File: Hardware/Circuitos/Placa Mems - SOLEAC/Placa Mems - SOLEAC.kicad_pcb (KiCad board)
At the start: 2 copper layers, 50 x 40 mm, 7 parts, among them J2 Conn_01x04, J6 Conn_01x02, Y1 MA40S4R

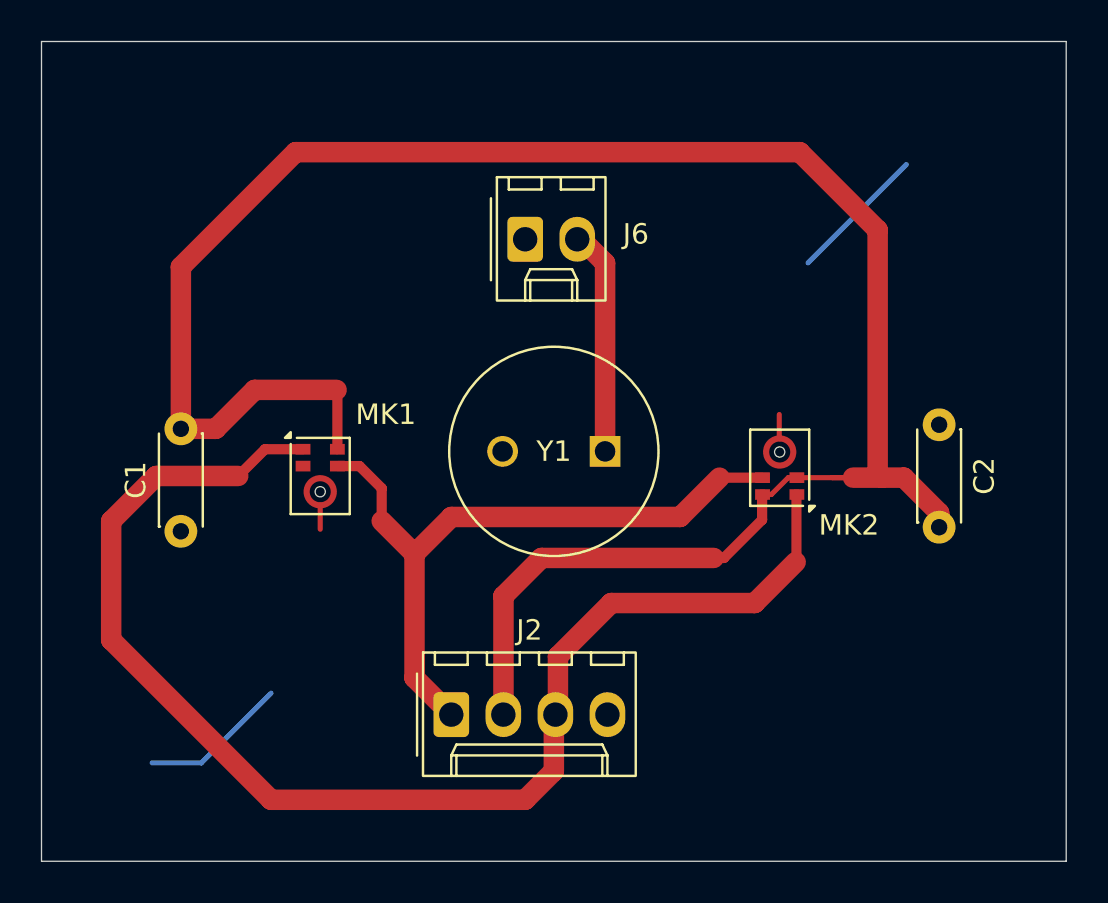
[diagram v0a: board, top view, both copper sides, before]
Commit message: Placa Mems - Zona de tierra
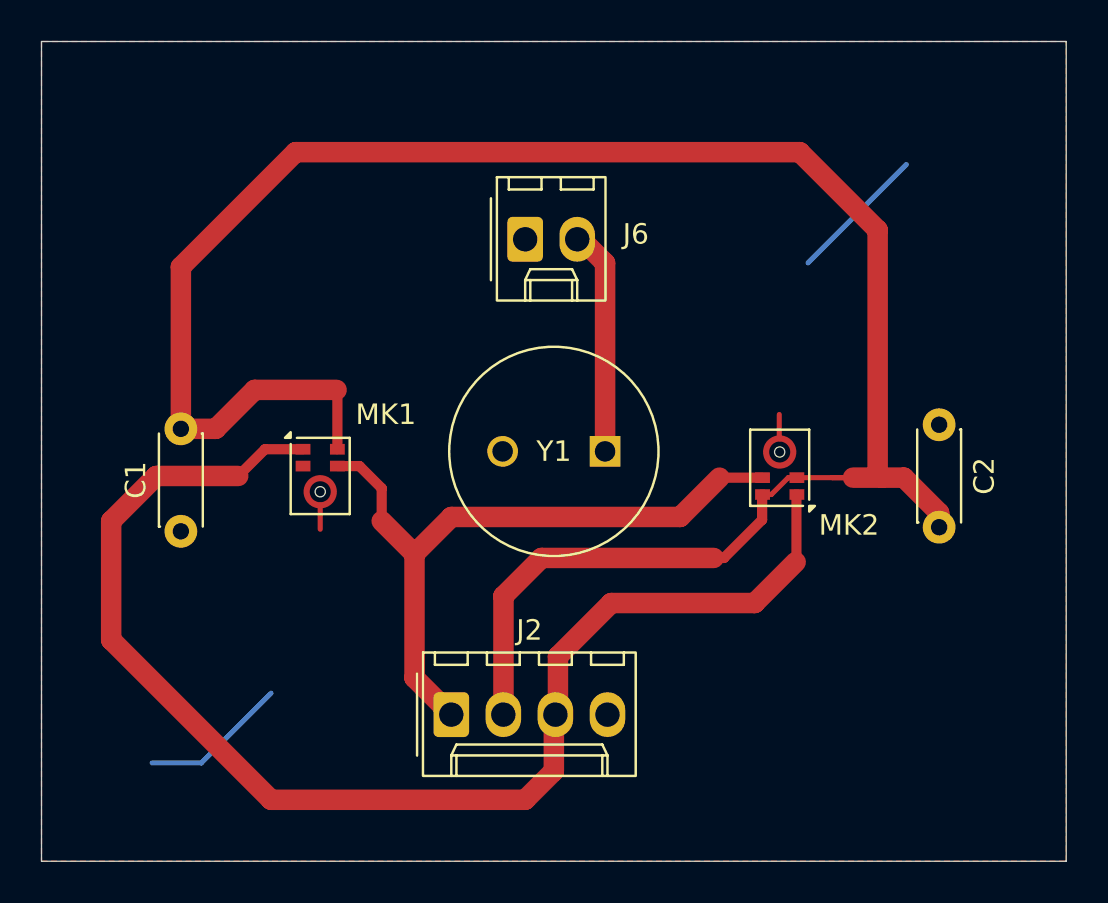
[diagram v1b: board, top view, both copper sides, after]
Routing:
- added copper zone on F.Cu, net Earth
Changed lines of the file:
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@@
 		(net "/entrada placa procesadora")
+	)
+	(zone
+		(net "Earth")
+		(layer "F.Cu")
+		(hatch edge 0.5)
+		(connect_pads
+			(clearance 0.5)
+		)
+		(min_thickness 0.25)
+		(fill yes
+			(thermal_gap 0.5)
+			(thermal_bridge_width 0.5)
+			(island_removal_mode 0)
+		)
+		(polygon
+			(pts
+				(xy 75.2 65.8) (xy 75.2 25.8) (xy 25.2 25.8) (xy 25.2 65.8)
+			)
+		)
 	)
 	(embedded_fonts no)
